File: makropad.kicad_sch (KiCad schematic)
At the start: 27 parts, among them J1 OLED_DISPLAY, SW1 SW_Push_45deg, SW10 SW_Push_45deg, SW11 RotaryEncoder_Switch, SW12 RotaryEncoder_Switch, SW2 SW_Push_45deg, SW3 SW_Push_45deg, SW4 SW_Push_45deg, SW5 SW_Push_45deg, SW6 SW_Push_45deg, SW7 SW_Push_45deg, SW8 SW_Push_45deg, SW9 SW_Push_45deg, U1 PCF8574A, U2 MOUDLE-SEEEDUINO-XIAO

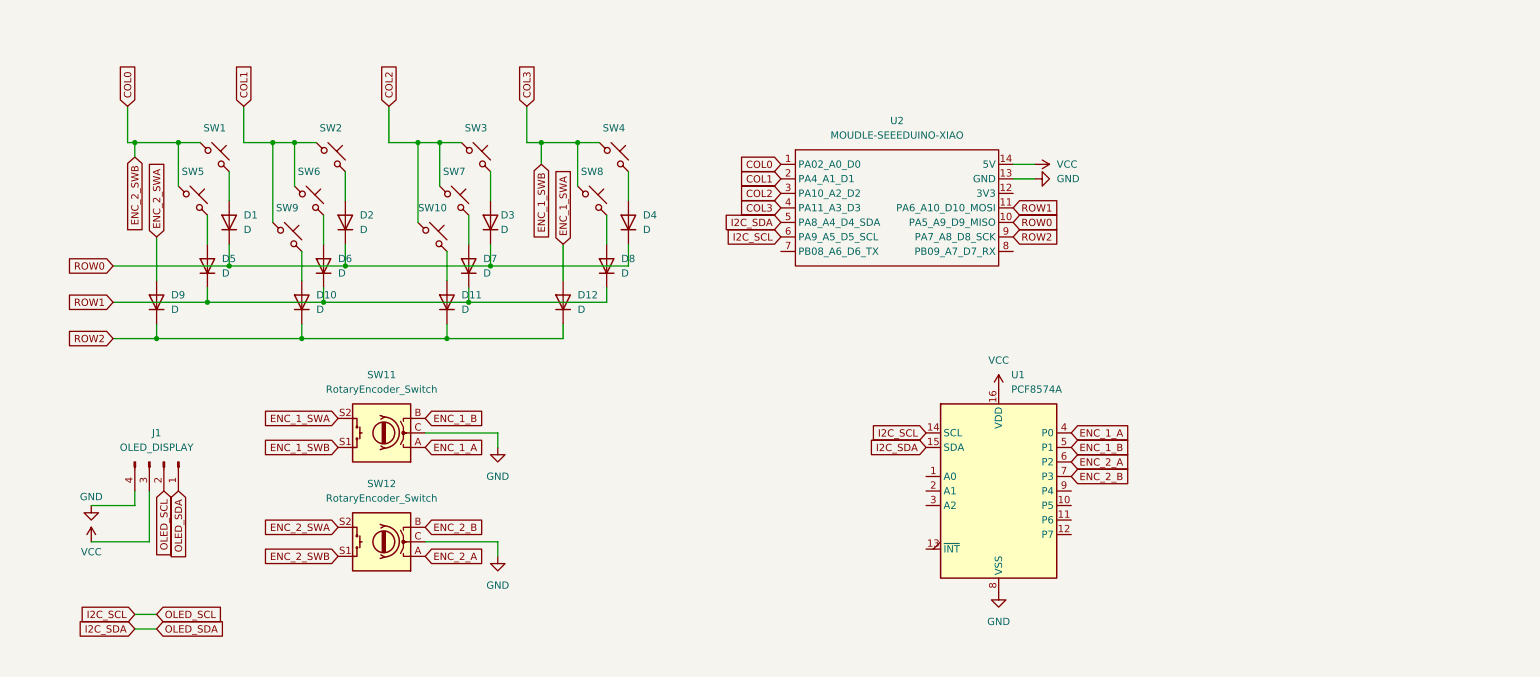
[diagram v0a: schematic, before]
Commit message: Finish pcb
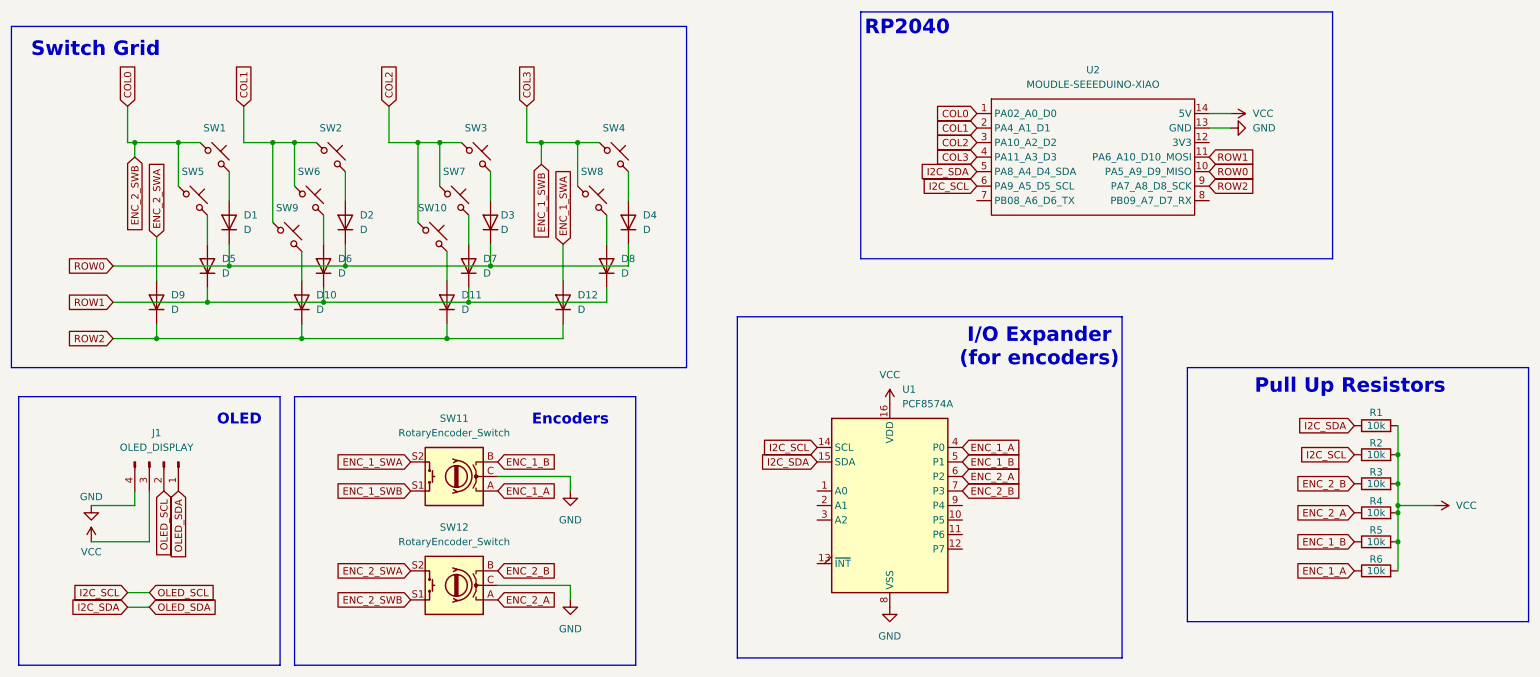
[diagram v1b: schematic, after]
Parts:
- added R1, R2, R3, R4, R5, R6: 10k, Resistor_SMD:R_1206_3216Metric, symbol Device:R
- D1, D10, D11, D12, D2, D3, D4, D5, D6, D7, D8, D9: footprint Diode_THT:D_DO-35_SOD27_P7.62mm_Horizontal -> Diode_SMD:D_1206_3216Metric
- J1: footprint Connector_PinHeader_2.54mm:PinHeader_1x04_P2.54mm_Vertical -> Components:SSD1306-0.91-OLED-4pin-128x32
- SW1, SW10, SW2, SW3, SW4, SW5, SW6, SW7, SW8, SW9: footprint MX_Solderable:MX-Solderable-1U -> Components:MX-Solderable-1U
- U1: footprint (none) -> Components:SOIC127P1032X265-16N
- U2: footprint (none) -> Components:XIAO-Generic-Hybrid-14P-2.54-21X17.8MM
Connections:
- net ENC_1_A: now also R6.1
- net ENC_1_B: now also R5.1
- net ENC_2_A: now also R4.1
- net ENC_2_B: now also R3.1
- net I2C_SCL: now also R2.1
- net I2C_SDA: now also R1.1
- net VCC: now also R1.2, R2.2, R3.2, R4.2, R5.2, R6.2
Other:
- note added: "Encoders"
- note added: "I/O Expander (for encoders)"
- note added: "OLED"
- note added: "Pull Up Resistors"
- note added: "RP2040"
- note added: "Switch Grid"
- moved on the sheet: SW11, SW12, U1, U2
